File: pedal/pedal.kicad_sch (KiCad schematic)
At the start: 8 parts, among them J1 AudioJack3, J2 AudioJack3, J3 Conn_01x08, J4 USB_B_Micro, U1 STM32H743ZGTx, U2 PCM3060, U3 LP2985-3.3, U4 TPS62170DSG

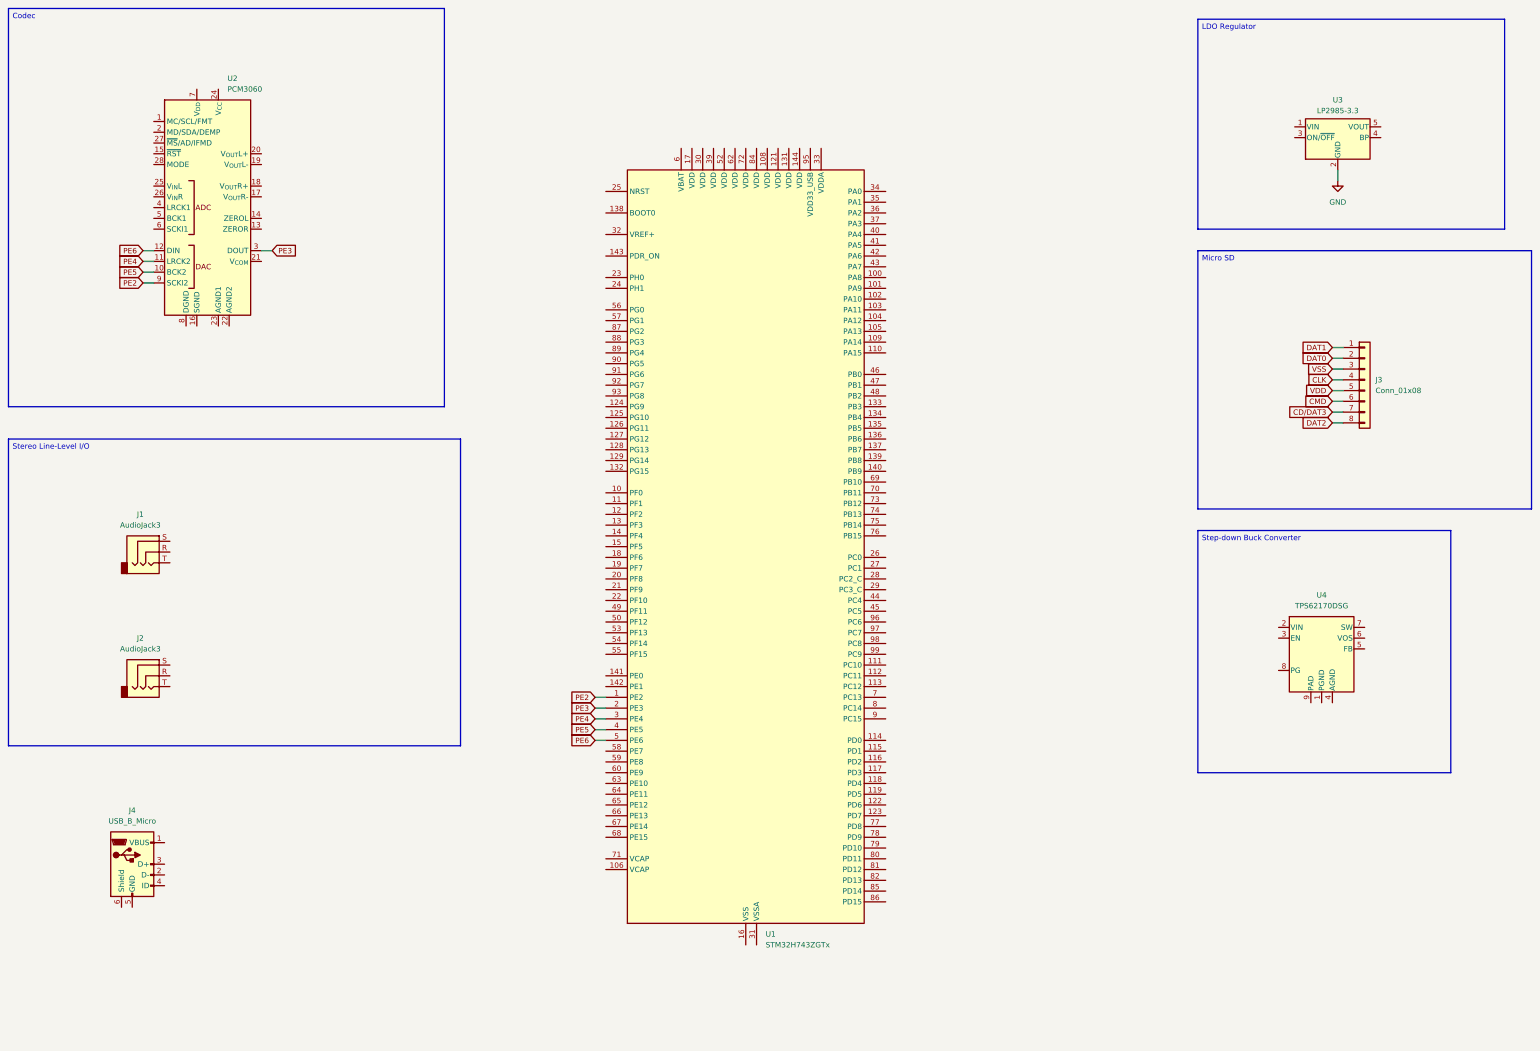
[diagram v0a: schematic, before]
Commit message: Update JOURNAL & DSP
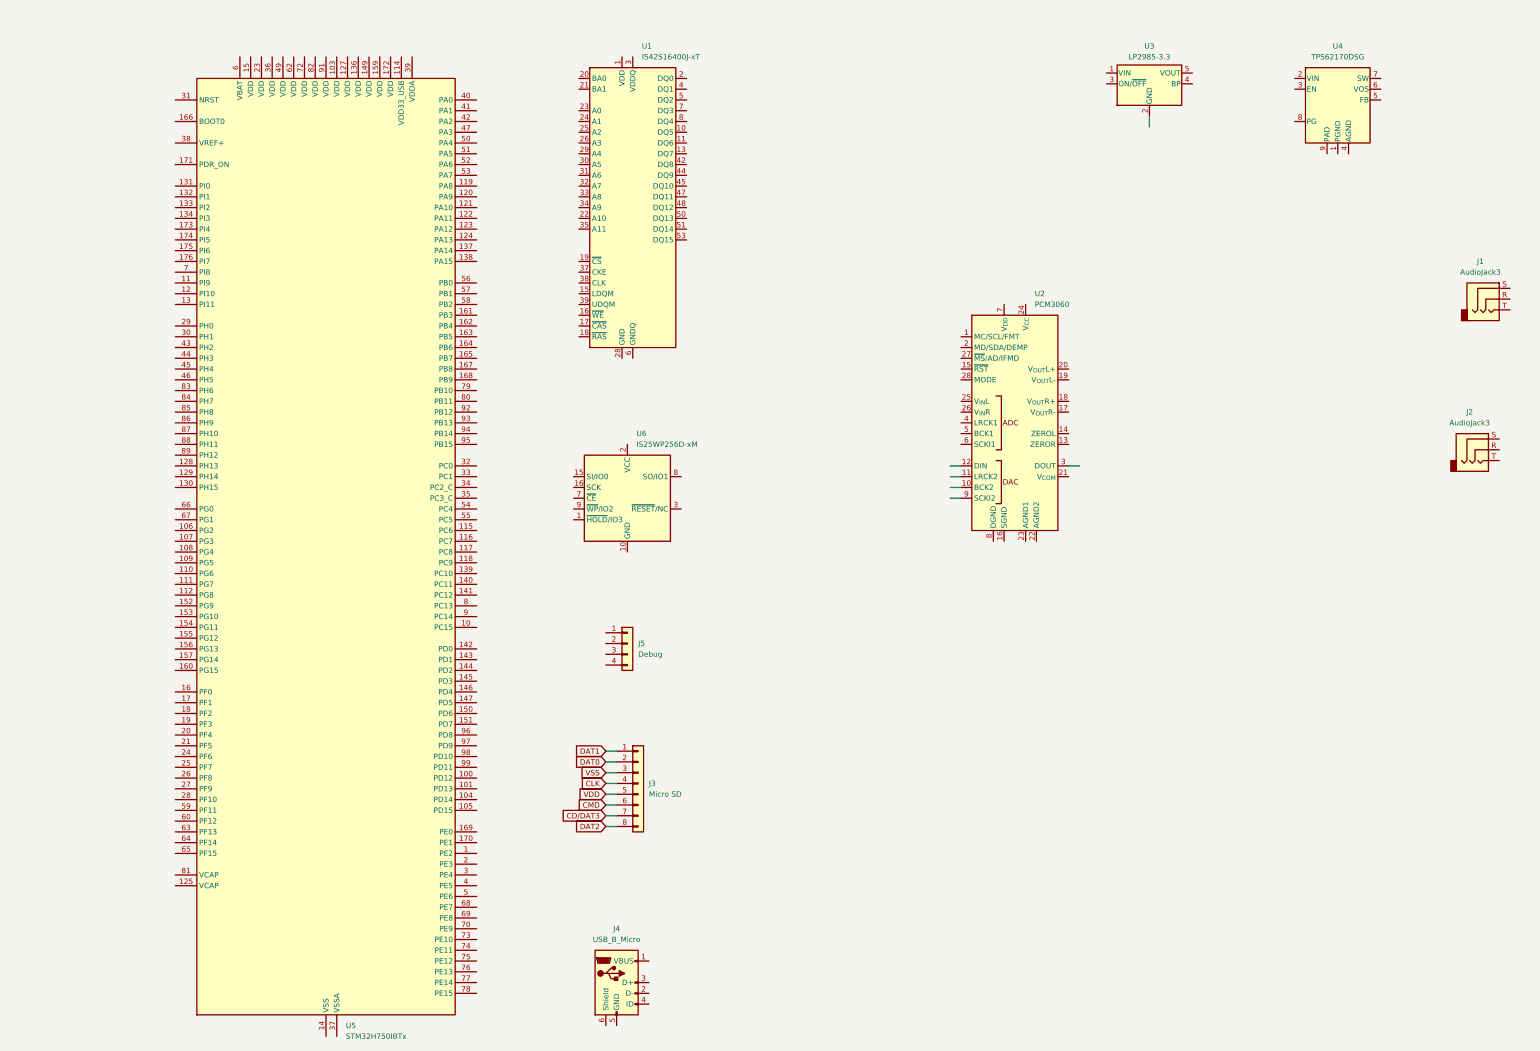
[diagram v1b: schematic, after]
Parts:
- removed U1: STM32H743ZGTx, Package_QFP:LQFP-144_20x20mm_P0.5mm, symbol MCU_ST_STM32H7:STM32H743ZGTx
- added J5: Debug, symbol Connector_Generic:Conn_01x04
- added U1: IS42S16400J-xT, Package_SO:TSOP-II-54_22.2x10.16mm_P0.8mm, symbol Memory_RAM:IS42S16400J-xT
- added U5: STM32H750IBTx, Package_QFP:LQFP-176_24x24mm_P0.5mm, symbol MCU_ST_STM32H7:STM32H750IBTx
- added U6: IS25WP256D-xM, Package_SO:SOIC-16W_7.5x10.3mm_P1.27mm, symbol Memory_Flash:IS25WP256D-xM
- J3: value Conn_01x08 -> Micro SD
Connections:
- net GND: no longer names the net of U3.2 (GND)
- net PE2: no longer names the net of U2.9 (SCKI2)
- net PE3: no longer names the net of U2.3 (DOUT)
- net PE4: no longer names the net of U2.11 (LRCK2)
- net PE5: no longer names the net of U2.10 (BCK2)
- net PE6: no longer names the net of U2.12 (DIN)
- new net: U1.1 (VDD), U1.14 (VDD), U1.27 (VDD)
- new net: U1.12 (GNDQ), U1.46 (GNDQ), U1.52 (GNDQ), U1.6 (GNDQ)
- new net: U1.28 (GND), U1.41 (GND), U1.54 (GND)
- new net: U1.3 (VDDQ), U1.43 (VDDQ), U1.49 (VDDQ), U1.9 (VDDQ)
- new net: U5.102 (VSS), U5.113 (VSS), U5.126 (VSS), U5.135 (VSS), U5.14 (VSS), U5.148 (VSS), U5.158 (VSS), U5.22 (VSS), U5.48 (VSS), U5.61 (VSS), U5.71 (VSS), U5.90 (VSS)
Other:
- moved on the sheet: J1, J2, J3, J4, U2, U3, U4
